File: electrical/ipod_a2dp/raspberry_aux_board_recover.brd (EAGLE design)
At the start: 100 x 80 mm, 33 parts, among them IC1 74LS244N

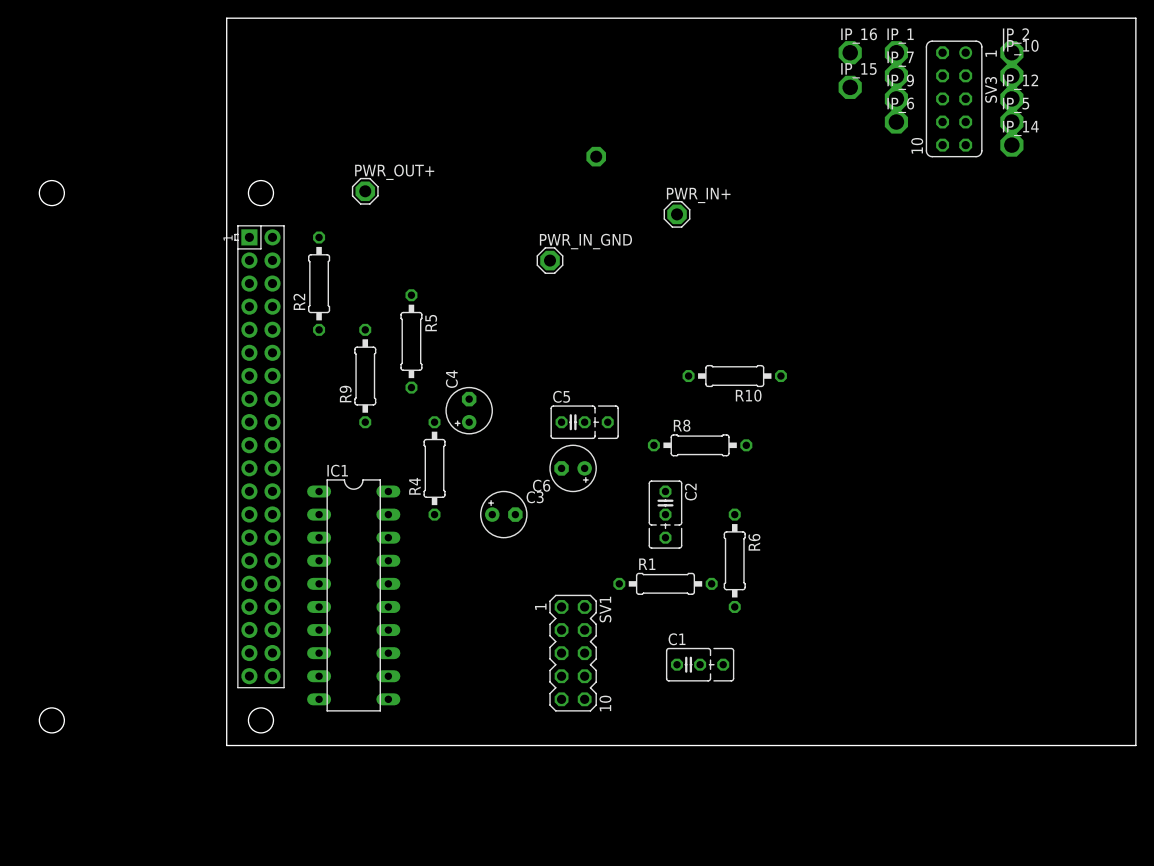
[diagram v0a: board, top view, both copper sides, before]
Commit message: updated board
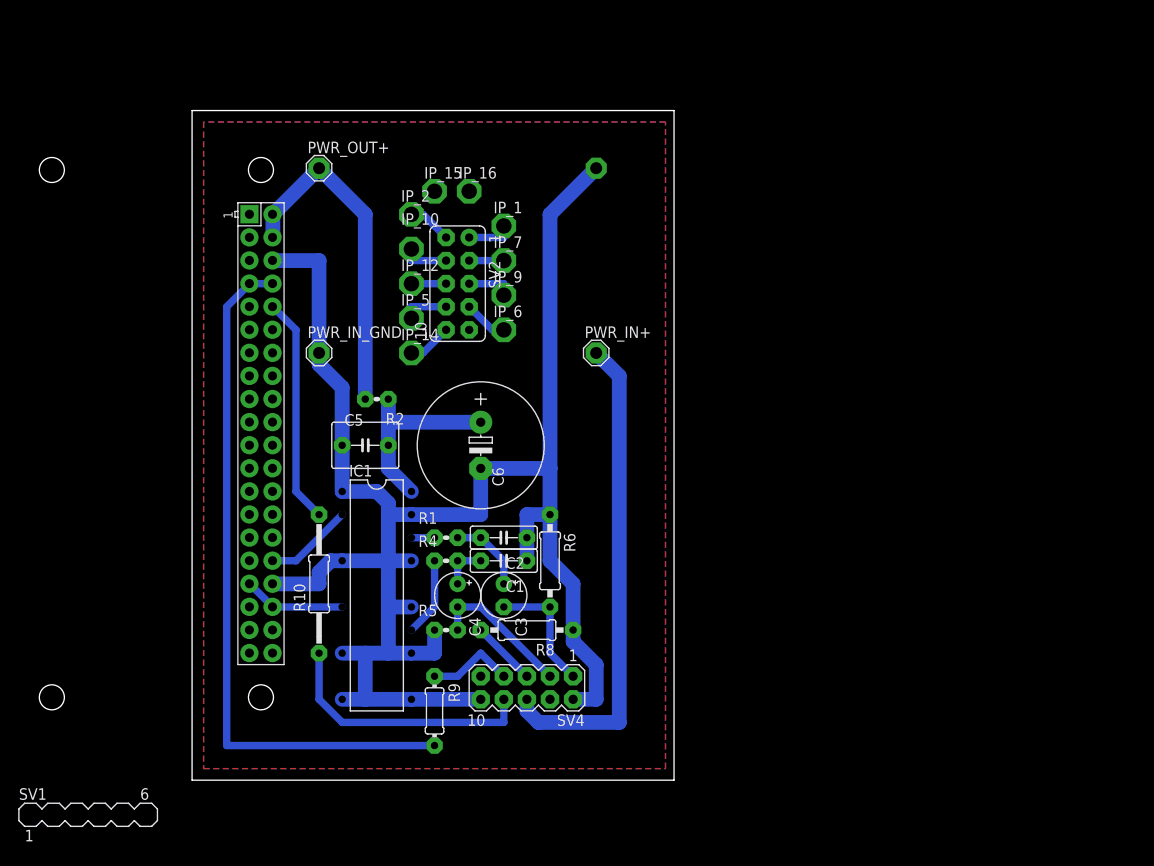
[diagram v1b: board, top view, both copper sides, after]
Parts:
- removed SV3: 10PIN_FEMALE, con-lsta:FE05-2
- added SV2: 10PIN_FEMALE, con-lsta:FE05-2
- added SV4: 10PIN_MALE, con-lstb:MA05-2
- C1, C2: device rcl:C025_050-035X075 -> rcl:C050-025X075
- C5: device rcl:C025_050-035X075 -> rcl:C050-050X075
- C6: device rcl:E2,5-5 -> rcl:E5-13
- R1, R2, R4, R5: device rcl:0207/10 -> rcl:0204V
- R10: device rcl:0207/10 -> rcl:0207/15
- R9: device rcl:0207/10 -> rcl:0204/7
- SV1: value 10PIN_MALE -> (none); device con-lstb:MA05-2 -> con-lstb:MA06-1
- moved IP_14 69.9 mm to (20.3, 43.2)
- moved IP_5 69.5 mm to (20.3, 47.0)
- moved IP_12 69.1 mm to (20.3, 50.8)
- moved IP_10 68.7 mm to (20.3, 54.6)
- moved IP_2 68.4 mm to (20.3, 58.4)
- moved SV1 56.2 mm to (-15.2, -7.62), turned to 0 degrees
- moved R10 51.1 mm to (10.2, 17.8), turned to 90 degrees
- moved IP_6 48.9 mm to (30.5, 45.7)
- moved IP_9 48.3 mm to (30.5, 49.5)
- moved IP_7 47.7 mm to (30.5, 53.3)
- moved IP_1 47.2 mm to (30.5, 57.1)
- moved IP_15 47.1 mm to (22.9, 61.0)
- moved IP_16 44.6 mm to (26.7, 61.0)
- moved R9 37.6 mm to (22.9, 3.81), turned to 270 degrees
- moved R5 32.0 mm to (24.1, 12.7), turned to 0 degrees
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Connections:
- net N$1 renamed PWM_AUDIO_R_OUT
- net N$4 renamed RPI_RX
- removed net N$2: R9.2, U$1.8
- removed net N$3: IC1.16, R4.1
- new net B_GND: SV1.1
- new net OR_TXD: SV1.4
- new net PWM_AUDIO_L_OUT: IC1.14, R4.1
- new net RPI_TX: R9.2, U$1.7, U$1.8
- new net Y_RXD: SV1.5
- net AUDIO_L: now also C4.-, R5.2, SV4.3; no longer C3.-, R6.2, SV1.4
- net AUDIO_L_DC: now also C1.2, C4.+, R4.2; no longer C2.2, C3.+, R1.2
- net AUDIO_L_OR: now also SV2.1; no longer SV3.2
- net AUDIO_R: now also C3.-, R6.2, SV4.1; no longer C4.-, R5.2, SV1.2
- net AUDIO_R_BR: now also SV2.3; no longer SV3.4
- net AUDIO_R_DC: now also C2.2, C3.+, R1.2; no longer C1.2, C4.+, R4.2
- net AUD_GND_B: now also SV2.2; no longer SV3.1
- net CHGR_PWR: now also SV4.6; no longer SV1.5
- net CHGR_PWR_B: now also SV2.6; no longer SV3.5
- net CONN_RECOG: now also SV4.5; no longer SV1.6
- net CONN_RECOG_Y: now also SV2.5; no longer SV3.6
- net GND: now also IC1.4, SV4.10, SV4.2; no longer IC1.6, SV1.1, SV1.9
- net IP_GND: now also SV2.4; no longer SV3.3
- net IP_RX: now also SV4.7; no longer SV1.8
- net IP_RX_P: now also SV2.7; no longer SV3.8
- net IP_TX: now also SV4.8; no longer SV1.7
- net IP_TX_GR: now also SV2.8; no longer SV3.7
- net PWM_AUD_L: now also IC1.6, U$1.33, U$1.36; no longer IC1.2, U$1.32
- net PWM_AUD_R: now also IC1.2, U$1.32; no longer IC1.4, U$1.33
- net SHIELD_RXTX_B: now also SV2.10; no longer SV3.9
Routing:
- net GND: track 0.00 -> 202.0 mm
- net RPI_TX: track 0.00 -> 77.3 mm
- net CHGR_PWR: track 0.00 -> 53.6 mm
- net VCC: track 0.00 -> 37.3 mm
- net IP_TX: track 0.00 -> 29.0 mm
- net RPI_RX: track 0.00 -> 25.0 mm
- net +5V0A: track 0.00 -> 21.4 mm
- net AUDIO_L: track 0.00 -> 15.9 mm
- net AUDIO_R: track 0.00 -> 13.8 mm
- net PWM_AUD_L: track 0.00 -> 11.3 mm
- net PWM_AUD_R: track 0.00 -> 9.77 mm
- net IP_RX: track 0.00 -> 9.72 mm
- net PWM_AUDIO_L_OUT: track 0.00 -> 8.67 mm
- net AUDIO_R_DC: track 0.00 -> 8.67 mm
- net CONN_RECOG: track 0.00 -> 7.18 mm
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- added copper zone on layer 1, net GND
- added copper zone on layer 16, net GND
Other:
- board size 100 x 80 mm -> 53 x 73.7 mm
- board text added: "jorgen@birkler.se"
